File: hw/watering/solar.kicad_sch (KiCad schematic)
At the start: 26 parts, among them U2 BQ25798

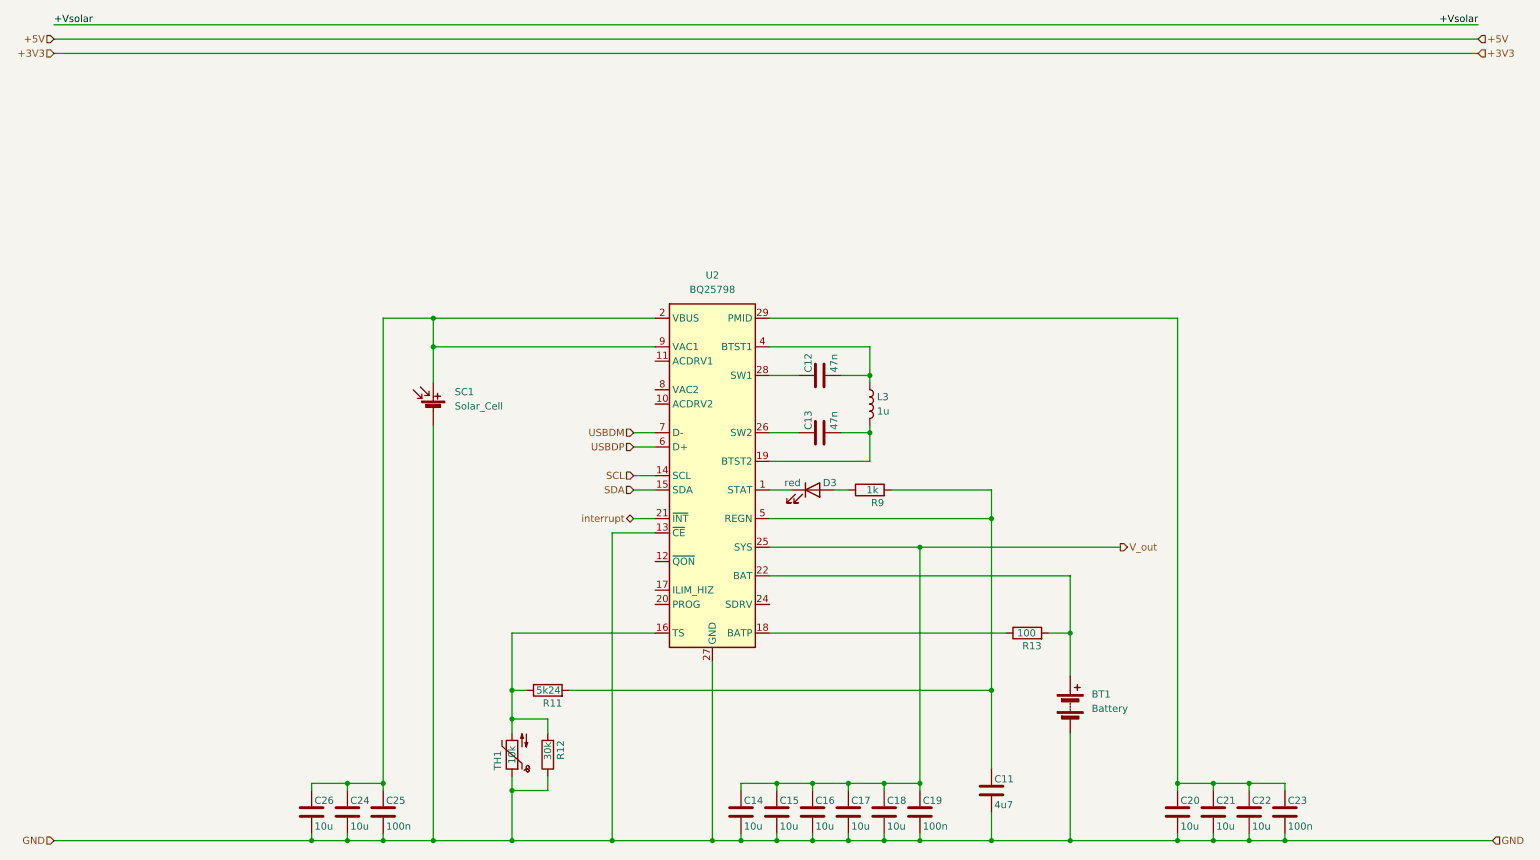
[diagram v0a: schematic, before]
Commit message: updated power
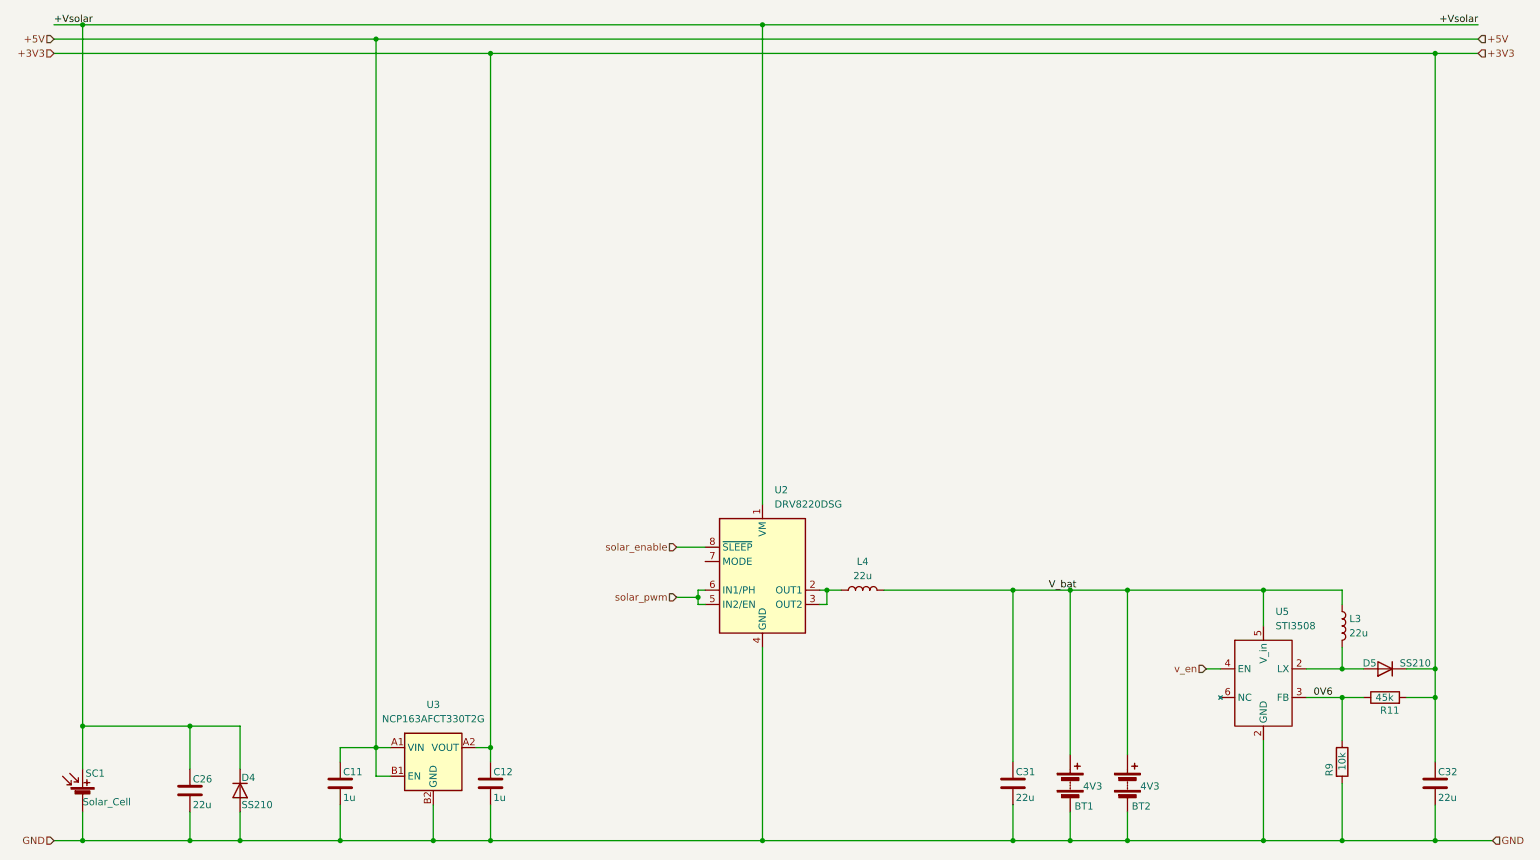
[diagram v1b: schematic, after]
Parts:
- removed C13: 47n, Capacitor_SMD:C_0603_1608Metric, symbol Device:C
- removed C14, C15, C16, C17, C18, C20, C21, C22, C24: 10u, Capacitor_SMD:C_0603_1608Metric, symbol Device:C
- removed C19, C23, C25: 100n, Capacitor_SMD:C_0603_1608Metric, symbol Device:C
- removed D3: red, symbol Device:LED
- removed R12: 30k, Resistor_SMD:R_0603_1608Metric, symbol Device:R
- removed R13: 100, Resistor_SMD:R_0603_1608Metric, symbol Device:R
- removed TH1: 10k, symbol Device:Thermistor_NTC
- removed U2: BQ25798, Package_DFN_QFN:Texas_RQM0029A_VQFN-29_4x4mm_P0.4mm, symbol Battery_Management:BQ25798
- added BT2: 4V3, batteryholder:BH-18650-B1BA002, symbol Device:Battery
- added C31, C32: 22u, Capacitor_SMD:C_1206_3216Metric, symbol Device:C
- added D4, D5: SS210, Diode_SMD:D_SMA, symbol Device:D
- added L4: 22u, Inductor_SMD:L_Wuerth_MAPI-4030, symbol Device:L
- added U2: DRV8220DSG, Package_SON:WSON-8-1EP_2x2mm_P0.5mm_EP0.9x1.6mm, symbol Driver_Motor:DRV8220DSG
- added U3: NCP163AFCT330T2G, Package_CSP:WLCSP-4_0.64x0.64mm_Layout2x2_P0.35mm, symbol Regulator_Linear:NCP163AFCT330T2G
- added U5: STI3508, Package_TO_SOT_SMD:SOT-23-6, symbol sti3508:STI3508
- BT1: value Battery -> 4V3; footprint Battery:BatteryHolder_Keystone_1042_1x18650 -> batteryholder:BH-18650-B1BA002
- C11: value 4u7 -> 1u
- C12: value 47n -> 1u
- C26: value 10u -> 22u; footprint Capacitor_SMD:C_0603_1608Metric -> Capacitor_SMD:C_1206_3216Metric
- L3: value 1u -> 22u; footprint (none) -> Inductor_SMD:L_Wuerth_MAPI-4030
- R11: value 5k24 -> 45k
- R9: value 1k -> 10k
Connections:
- net +3V3: now also C12.1, R11.2, C32.1, D5.1 (K), U3.A2 (VOUT)
- net +5V: now also C11.1, U3.A1 (VIN), U3.B1 (EN)
- net +Vsolar: now also C26.1, SC1.1 (+), D4.1 (K), U2.1 (VM)
- net GND: now also C12.2, R9.2, BT2.2 (-), C31.2, C32.2, D4.2 (A), U2.4 (GND), U2.9 (GND), U3.B2 (GND), U5.2 (LX)
- net V_bat: now reaches L3.1
- net V_bat: now also BT1.1 (+), BT2.1 (+), C31.1, L4.2, U5.5 (V_in); no longer C12.2
- net 0V6: now reaches R9.1
- net 0V6: now also R11.1, U5.3 (FB)
- net at L3.2: now also D5.2 (A), U5.2 (LX)
- new net: L4.1, U2.2 (OUT1), U2.3 (OUT2)
- new net solar_enable: U2.8 (~{SLEEP})
- new net solar_pwm: U2.5 (IN2/EN), U2.6 (IN1/PH)
- new net v_en: U5.4 (EN)
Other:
- moved on the sheet: BT1, C26, SC1
